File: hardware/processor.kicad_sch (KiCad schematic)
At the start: 1 part, among them U1 68LC040

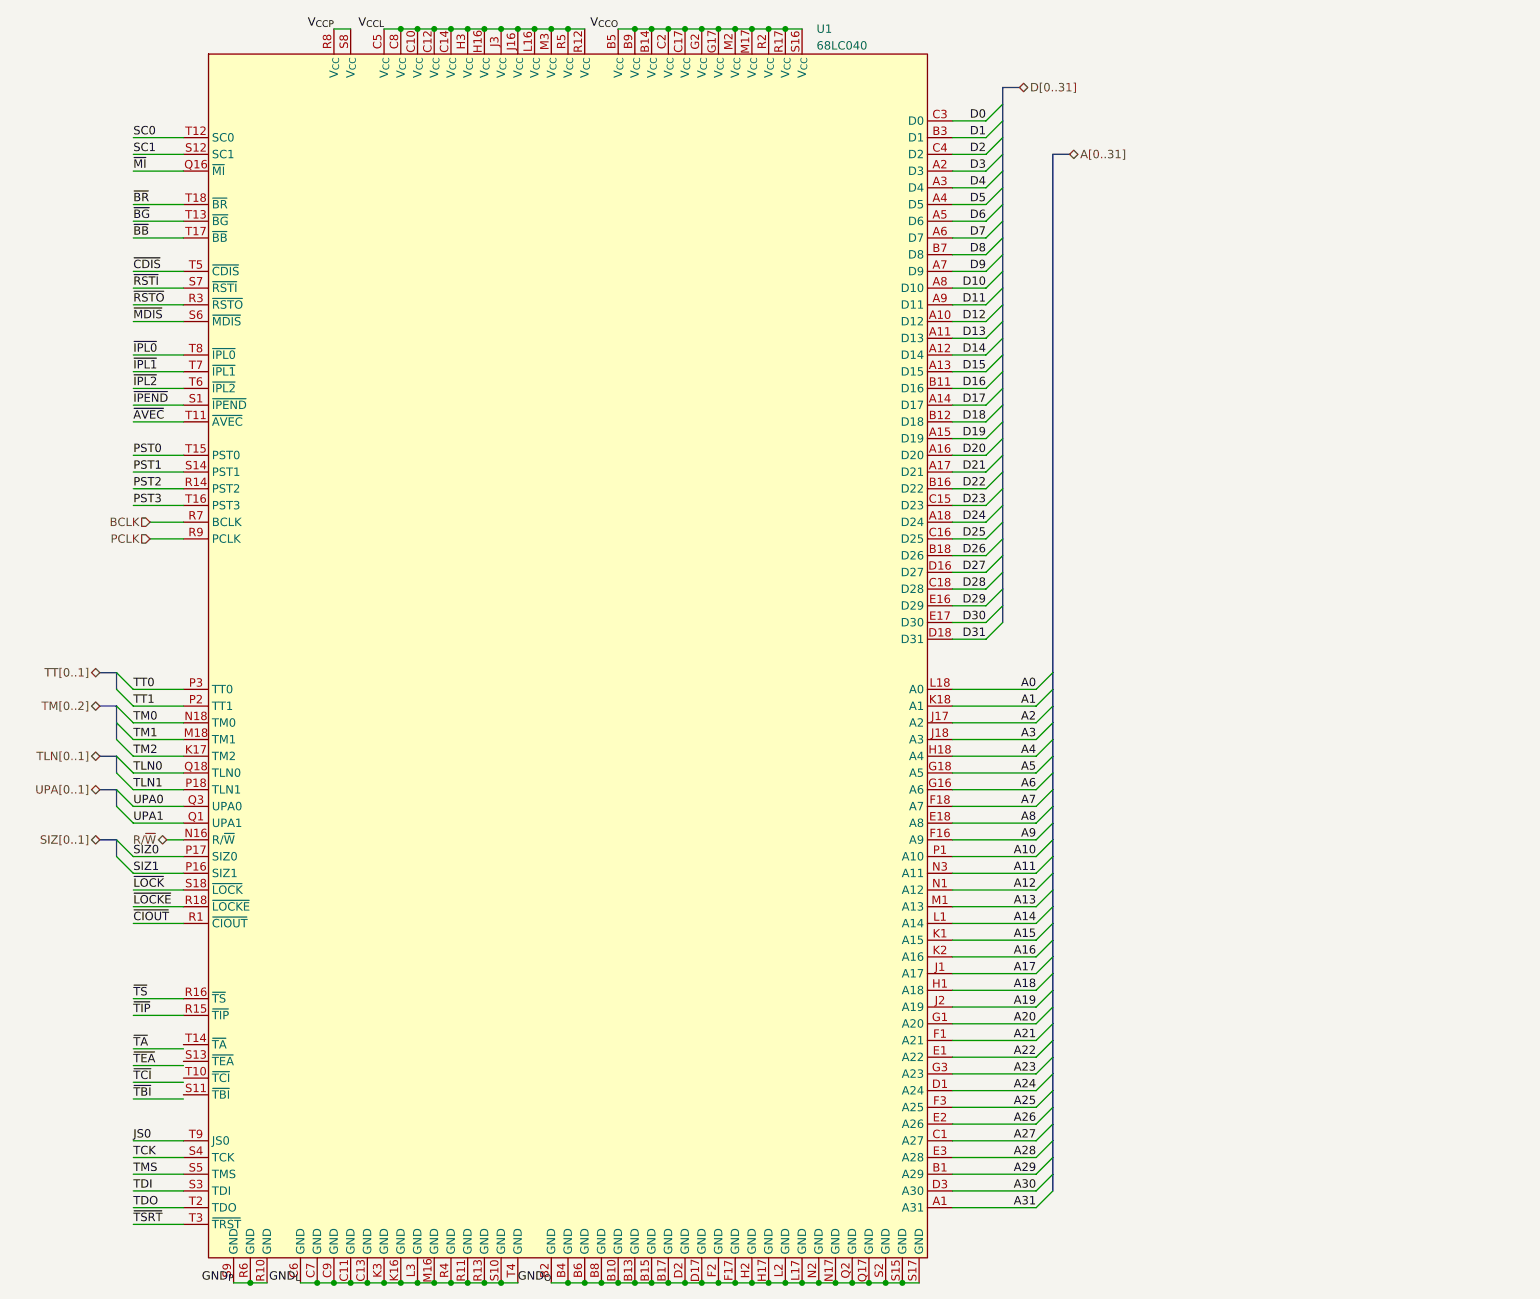
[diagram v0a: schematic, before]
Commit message: update cpu symbol, topology
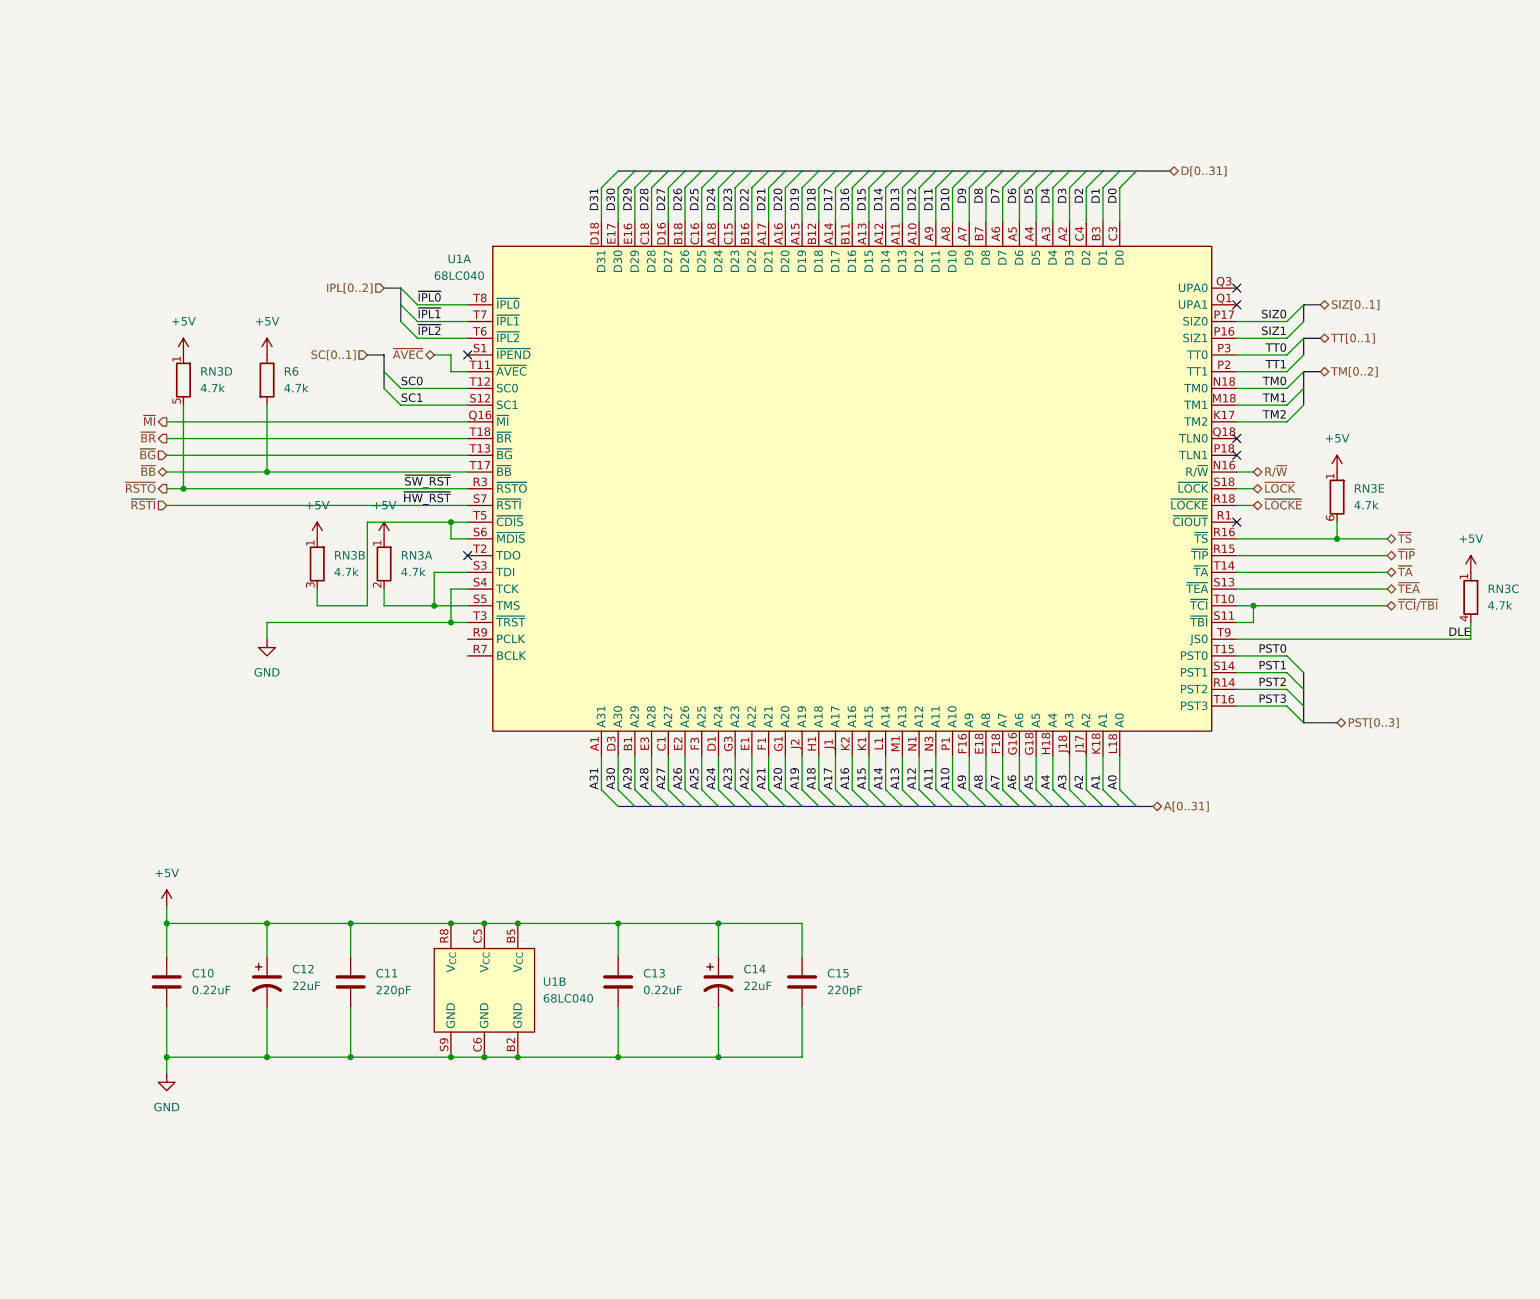
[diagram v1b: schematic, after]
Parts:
- added C10, C13: 0.22uF, symbol Device:C
- added C11, C15: 220pF, symbol Device:C
- added C12, C14: 22uF, symbol Device:C_Polarized_US
- added R6: 4.7k, symbol Device:R
- added RN3: 4.7k, Resistor_THT:R_Array_SIP6, symbol Device:R_Network05_Split
- added unit 2 of U1
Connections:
- net TMS is gone; now on an unnamed net: U1.S5 (TMS)
- net ~{MDIS} is gone; now on an unnamed net: U1.S6 (~{MDIS})
- net ~{TSRT} is gone; now on net GND: U1.T3 (~{TRST})
- net ~{BB}: now also R6.2
- net ~{RSTO}: now also RN3.5 (R4.2)
- net ~{TA}: now also U1.T14 (~{TA})
- net ~{TEA}: now also U1.S13 (~{TEA})
- net ~{TS}: now also RN3.6 (R5.2)
- net ~{TCI}/~{TBI}: now reaches U1.S11 (~{TBI})
- net ~{TCI}/~{TBI}: now also U1.T10 (~{TCI})
- net BCLK: no longer names the net of U1.R7 (BCLK)
- removed net GND_{L}: U1.C11 (GND), U1.C13 (GND), U1.C6 (GND), U1.C7 (GND), U1.C9 (GND), U1.K16 (GND), U1.K3 (GND), U1.L3 (GND), U1.M16 (GND), U1.R11 (GND), U1.R13 (GND), U1.R4 (GND), U1.S10 (GND), U1.T4 (GND)
- removed net GND_{O}: U1.B10 (GND), U1.B13 (GND), U1.B15 (GND), U1.B17 (GND), U1.B2 (GND), U1.B4 (GND), U1.B6 (GND), U1.B8 (GND), U1.D17 (GND), U1.D2 (GND), U1.F17 (GND), U1.F2 (GND), U1.H17 (GND), U1.H2 (GND), U1.L17 (GND), U1.L2 (GND), U1.N17 (GND), U1.N2 (GND), U1.Q17 (GND), U1.Q2 (GND), U1.S15 (GND), U1.S17 (GND), U1.S2 (GND)
- removed net GND_{P}: U1.R10 (GND), U1.R6 (GND), U1.S9 (GND)
- net JS0 renamed DLE
- net DLE: now also RN3.4 (R3.2)
- net PCLK: no longer names the net of U1.R9 (PCLK)
- net TCK renamed GND
- net GND: now also C10.2, C11.2, C12.2, C13.2, C14.2, C15.2, U1.B10 (GND), U1.B13 (GND), U1.B15 (GND), U1.B17 (GND), U1.B2 (GND), U1.B4 (GND), U1.B6 (GND), U1.B8 (GND), U1.C11 (GND), U1.C13 (GND), U1.C6 (GND), U1.C7 (GND), U1.C9 (GND), U1.D17 (GND), U1.D2 (GND), U1.F17 (GND), U1.F2 (GND), U1.H17 (GND), U1.H2 (GND), U1.K16 (GND), U1.K3 (GND), U1.L17 (GND), U1.L2 (GND), U1.L3 (GND), U1.M16 (GND), U1.N17 (GND), U1.N2 (GND), U1.Q17 (GND), U1.Q2 (GND), U1.R10 (GND), U1.R11 (GND), U1.R13 (GND), U1.R4 (GND), U1.R6 (GND), U1.S10 (GND), U1.S15 (GND), U1.S17 (GND), U1.S2 (GND), U1.S9 (GND), U1.T4 (GND)
- net TDI: no longer names the net of U1.S3 (TDI)
- net TDI: now also RN3.2 (R1.2)
- net TDO: no longer names the net of U1.T2 (TDO)
- net TLN0: no longer names the net of U1.Q18 (TLN0)
- net TLN1: no longer names the net of U1.P18 (TLN1)
- net UPA0: no longer names the net of U1.Q3 (UPA0)
- net UPA1: no longer names the net of U1.Q1 (UPA1)
- removed net V_{CC}_{L}: U1.C10 (V_{CC}), U1.C12 (V_{CC}), U1.C14 (V_{CC}), U1.C5 (V_{CC}), U1.C8 (V_{CC}), U1.H16 (V_{CC}), U1.H3 (V_{CC}), U1.J16 (V_{CC}), U1.J3 (V_{CC}), U1.L16 (V_{CC}), U1.M3 (V_{CC}), U1.R12 (V_{CC}), U1.R5 (V_{CC})
- removed net V_{CC}_{O}: U1.B14 (V_{CC}), U1.B5 (V_{CC}), U1.B9 (V_{CC}), U1.C17 (V_{CC}), U1.C2 (V_{CC}), U1.G17 (V_{CC}), U1.G2 (V_{CC}), U1.M17 (V_{CC}), U1.M2 (V_{CC}), U1.R17 (V_{CC}), U1.R2 (V_{CC}), U1.S16 (V_{CC})
- removed net V_{CC}_{P}: U1.R8 (V_{CC}), U1.S8 (V_{CC})
- net ~{CDIS}: no longer names the net of U1.T5 (~{CDIS})
- net ~{CDIS}: now also RN3.3 (R2.2)
- net ~{CIOUT}: no longer names the net of U1.R1 (~{CIOUT})
- net ~{IPEND}: no longer names the net of U1.S1 (~{IPEND})
- new net +5V: C10.1, C11.1, C12.1, C13.1, C14.1, C15.1, R6.1, RN3.1 (R1), RN3.1 (R1), RN3.1 (R1), RN3.1 (R1), RN3.1 (R1), U1.B14 (V_{CC}), U1.B5 (V_{CC}), U1.B9 (V_{CC}), U1.C10 (V_{CC}), U1.C12 (V_{CC}), U1.C14 (V_{CC}), U1.C17 (V_{CC}), U1.C2 (V_{CC}), U1.C5 (V_{CC}), U1.C8 (V_{CC}), U1.G17 (V_{CC}), U1.G2 (V_{CC}), U1.H16 (V_{CC}), U1.H3 (V_{CC}), U1.J16 (V_{CC}), U1.J3 (V_{CC}), U1.L16 (V_{CC}), U1.M17 (V_{CC}), U1.M2 (V_{CC}), U1.M3 (V_{CC}), U1.R12 (V_{CC}), U1.R17 (V_{CC}), U1.R2 (V_{CC}), U1.R5 (V_{CC}), U1.R8 (V_{CC}), U1.S16 (V_{CC}), U1.S8 (V_{CC})
- no-connect marks 0 -> 7
